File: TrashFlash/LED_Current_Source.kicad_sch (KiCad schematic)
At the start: 22 parts, among them IC3 OPA191IDBVR, Q1 BC56-10PA,115, Q2 BC56-10PA,115, Q3 BC56-10PA,115, Q4 BC56-10PA,115

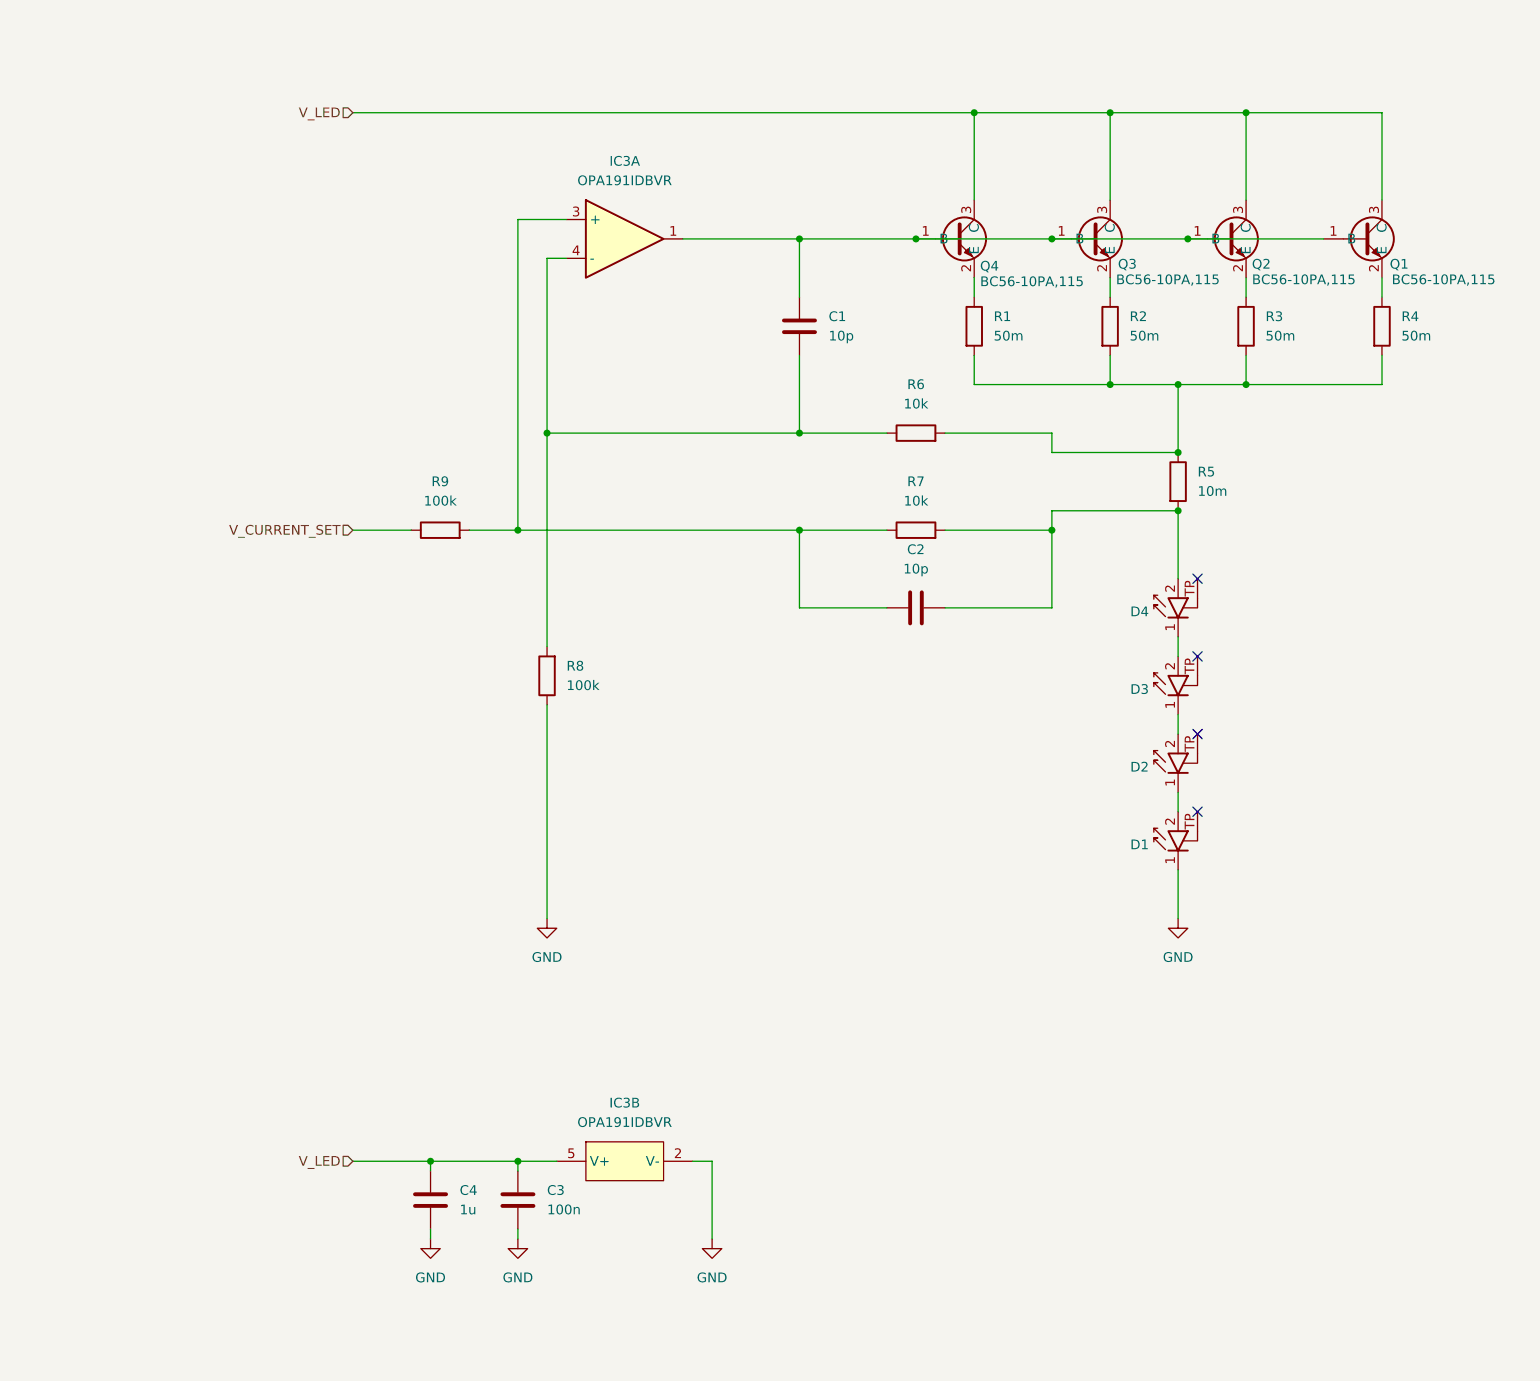
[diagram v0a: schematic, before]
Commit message: Started redrawing shematic
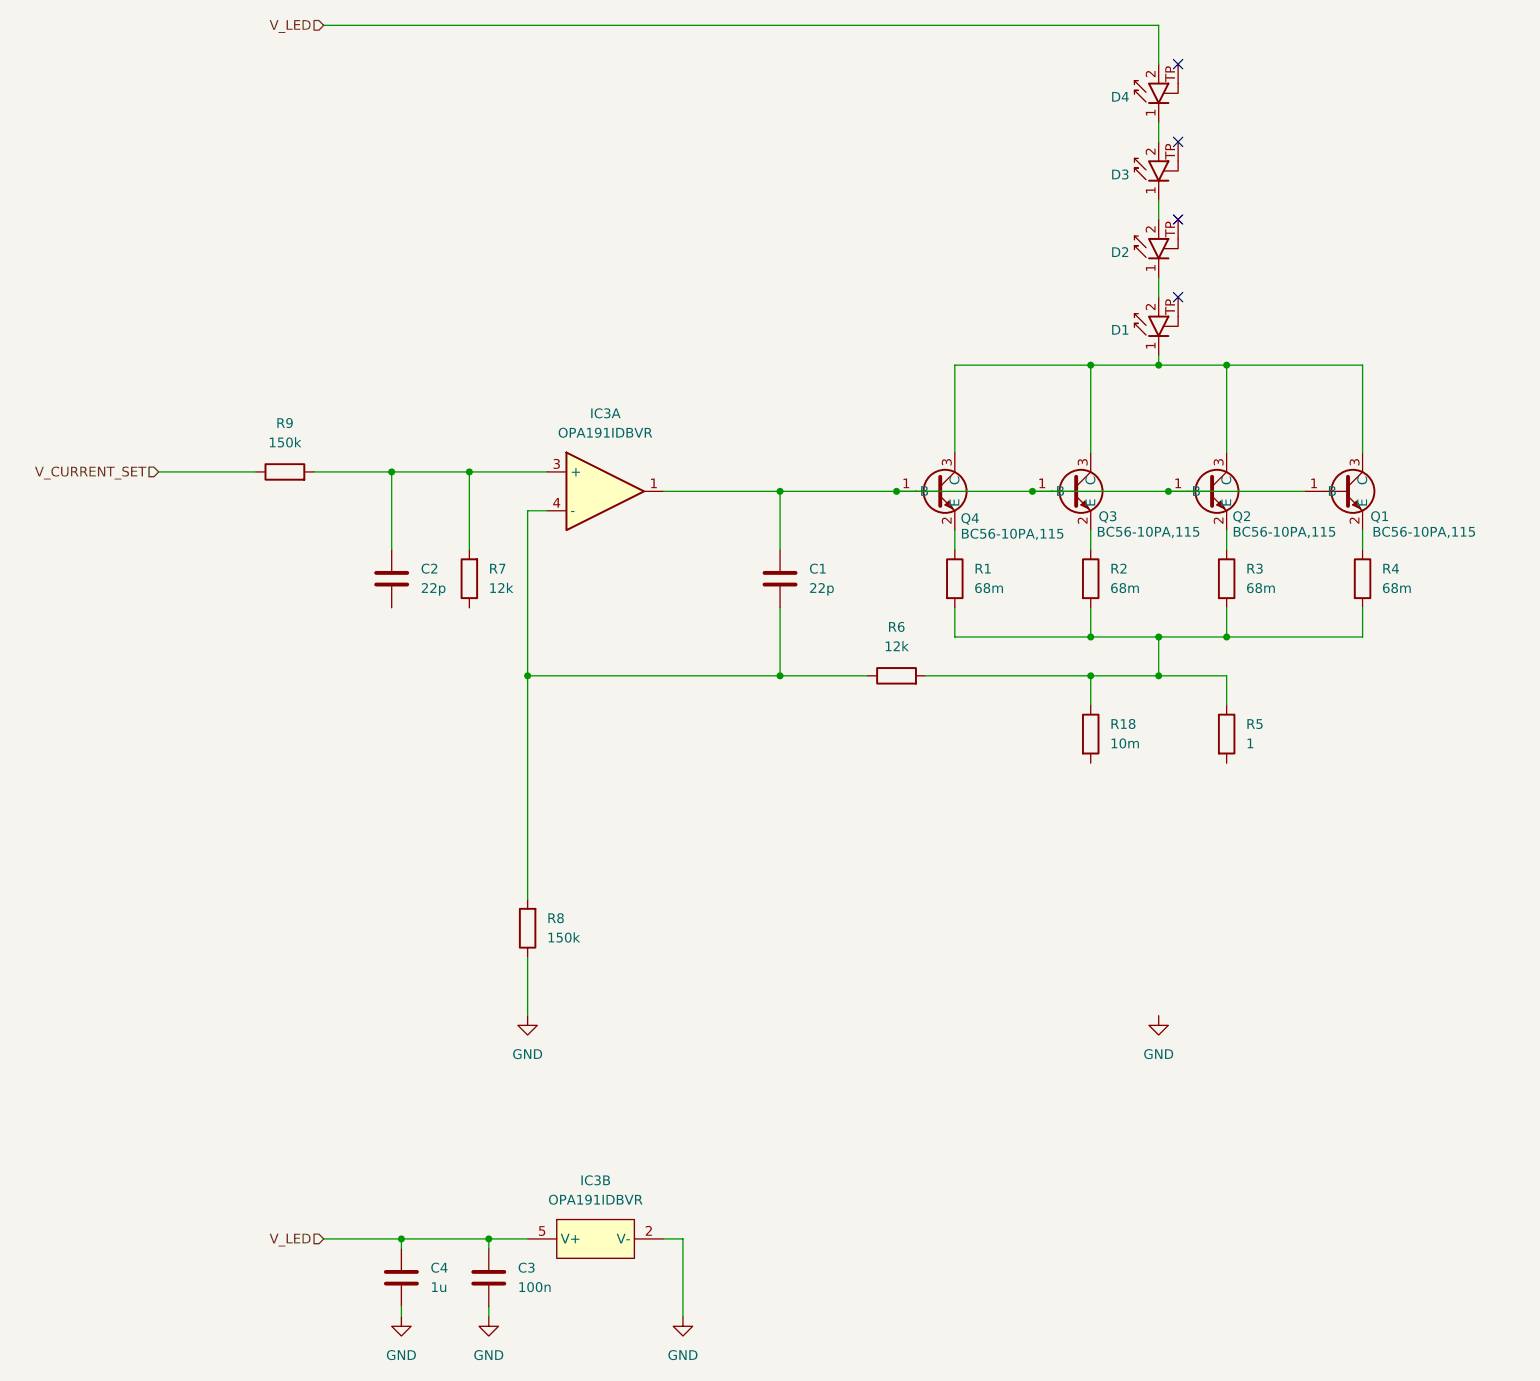
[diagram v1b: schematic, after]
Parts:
- added R18: 10m, symbol Device:R
- C1, C2: value 10p -> 22p
- R1, R2, R3, R4: value 50m -> 68m; footprint (none) -> Resistor_SMD:R_0603_1608Metric
- R5: value 10m -> 1
- R6, R7: value 10k -> 12k
- R8, R9: value 100k -> 150k
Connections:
- net GND: no longer D1.1 (K)
- net V_LED: now also D4.2 (A); no longer Q1.3 (C), Q2.3 (C), Q3.3 (C), Q4.3 (C)
- net at R1.2, R2.2, R3.2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: now also R18.1
- net at IC3.3 (+), R9.2: now also C2.2, R7.2; no longer C2.1, R7.1
- new net: D1.1 (K), Q1.3 (C), Q2.3 (C), Q3.3 (C), Q4.3 (C)
- now unconnected: R5.2
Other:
- moved on the sheet: C1, C2, C3, C4, D1, D2, D3, D4, IC3A, IC3B, Q1, Q2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
